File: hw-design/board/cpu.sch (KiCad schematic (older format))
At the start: 22 parts, among them P1 CHAIN, P2 USB_OTG, P3 CONN_02X05, Q7 BC857, SW1 SW_PUSH, U4 LPC11U24FBD48/401, Y1 12MHz

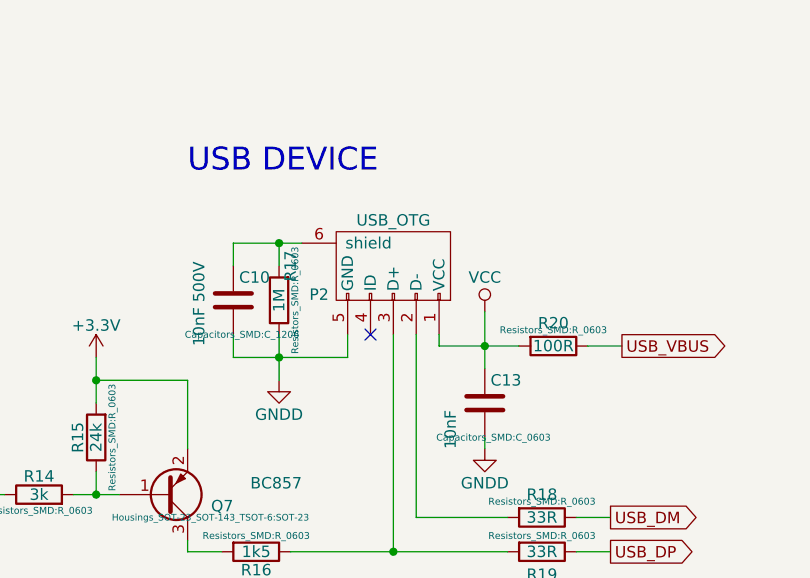
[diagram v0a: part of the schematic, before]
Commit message: sch: setting footprints and updating BOM
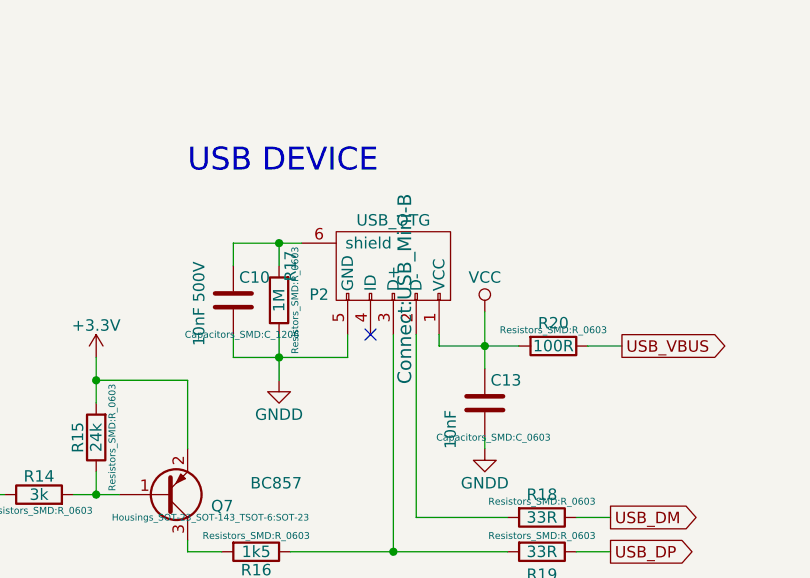
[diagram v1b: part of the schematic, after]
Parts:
- P2: footprint (none) -> Connect:USB_Mini-B
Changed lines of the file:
@@
 F 0 "P2" H 3675 5975 50  0000 C CNN
 F 1 "USB_OTG" H 3350 6300 50  0000 C CNN
-F 2 "" V 3300 6000 60  0000 C CNN
+F 2 "Connect:USB_Mini-B" V 3300 6000 60  0000 C CNN
 F 3 "" V 3300 6000 60  0000 C CNN
 F 4 "10033526-N3212LF" H 0   0   50  0001 C CNN "MPN"
